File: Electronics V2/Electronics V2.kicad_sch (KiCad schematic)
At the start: 57 parts, among them J1 MOT_L, J2 MOT_R, J3 SD_Card, J4 USB_C_Receptacle_USB2.0_14P, SW1 BTN_0, SW3 RST, SW4 BOOT, SW5 BTN_1, SW6 BTN_2, SW7 BTN_3, SW8 INCR_0, U1 NCP1117-3.3_SOT223, U10 TVS1400DRV, U11 TVS1400DRV, U3 ESP32-S3-WROOM-1, U4 DAC081C081CIMK, U5 IMU_L, U6 IMU_R, U7 NCP1117-3.3_SOT223, U8 SSD1036

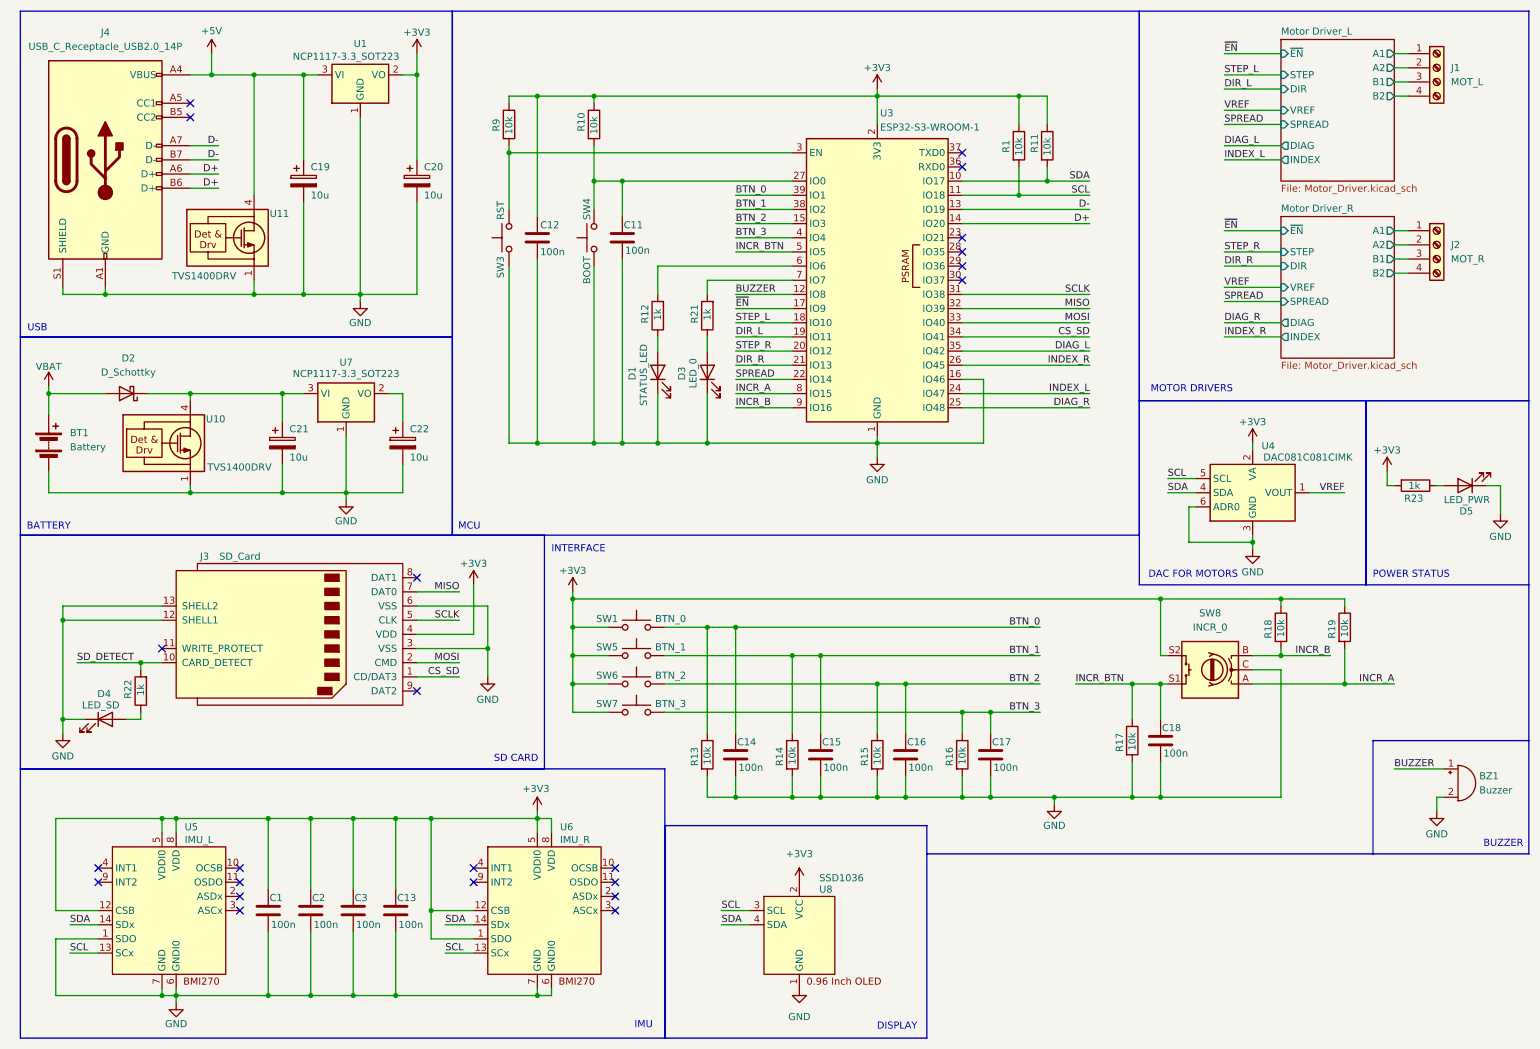
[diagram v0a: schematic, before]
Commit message: ready ro route
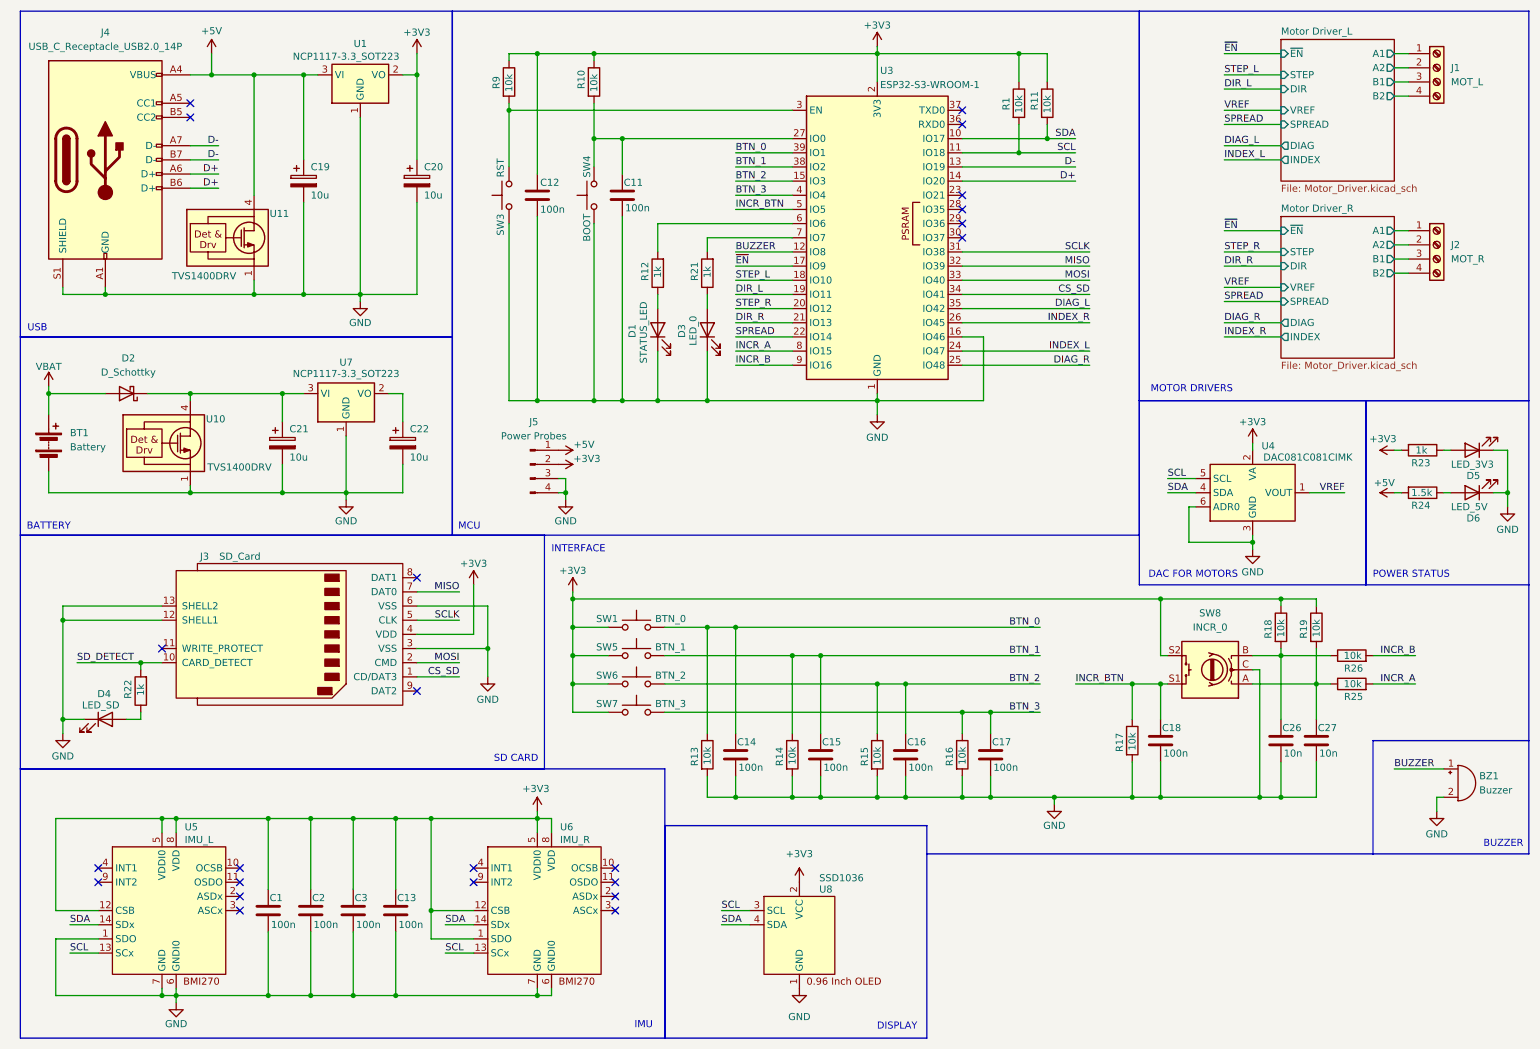
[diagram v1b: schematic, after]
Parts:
- added C26, C27: 10n, Capacitor_SMD:C_0603_1608Metric, symbol Device:C
- added D6: LED_5V, LED_SMD:LED_0603_1608Metric, symbol Device:LED
- added J5: Power Probes, Connector_PinHeader_2.54mm:PinHeader_1x04_P2.54mm_Vertical, symbol Connector:Conn_01x04_Pin
- added R24: 1.5k, Resistor_SMD:R_0603_1608Metric, symbol Device:R
- added R25, R26: 10k, Resistor_SMD:R_0603_1608Metric, symbol Device:R
- D2: footprint (none) -> Rotary_Encoder:RotaryEncoder_Bourns_Vertical_PEC12R-3x17F-Sxxxx
- D5: value LED_PWR -> LED_3V3
- J4: footprint Connector_Card:SD_TE_2041021 -> Connector_USB:USB_C_Receptacle_GCT_USB4110
- SW8: footprint Connector_Card:SD_Hirose_DM1AA_SF_PEJ82 -> Rotary_Encoder:RotaryEncoder_Bourns_Vertical_PEC12R-3x17F-Sxxxx
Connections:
- net +3V3: now also J5.2 (Pin_2)
- net +5V: now also J5.1 (Pin_1), R24.2
- net GND: now also C26.2, C27.2, D6.1 (K), J5.3 (Pin_3), J5.4 (Pin_4)
- net INCR_A: now also R25.2; no longer R19.2, SW8.A
- net INCR_B: now also R26.2; no longer R18.2, SW8.B
- new net: C27.1, R19.2, R25.1, SW8.A
- new net: D6.2 (A), R24.1
- new net: C26.1, R18.2, R26.1, SW8.B
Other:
- moved on the sheet: C11, C12, D1, D3, D5, R1, R10, R11, R12, R19, R21, R23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
